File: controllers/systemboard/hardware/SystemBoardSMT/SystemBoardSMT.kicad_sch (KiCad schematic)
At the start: 35 parts, among them J1 5V, J2 5V, J3 JTAG, SW1 RESET, U1 ATF1508AS-xxAx100, U2 74HC14, Y1 Crystal

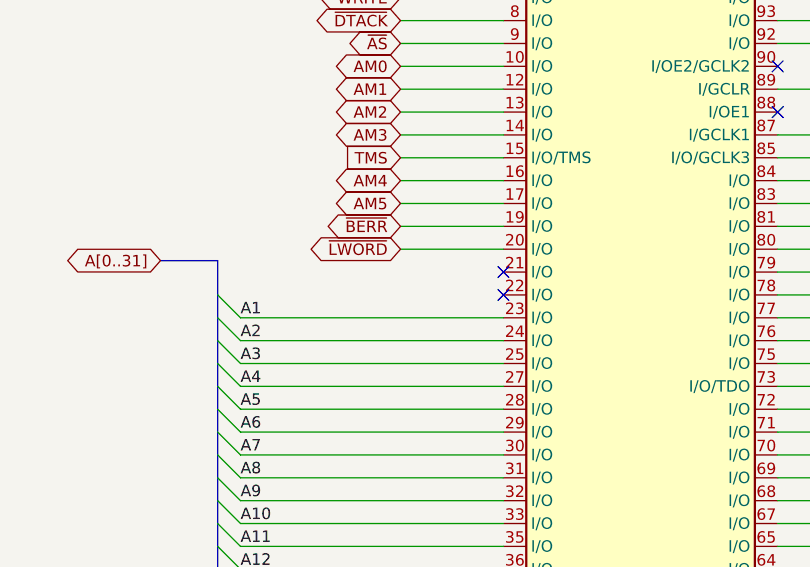
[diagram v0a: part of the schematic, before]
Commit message: Reorganized a bit
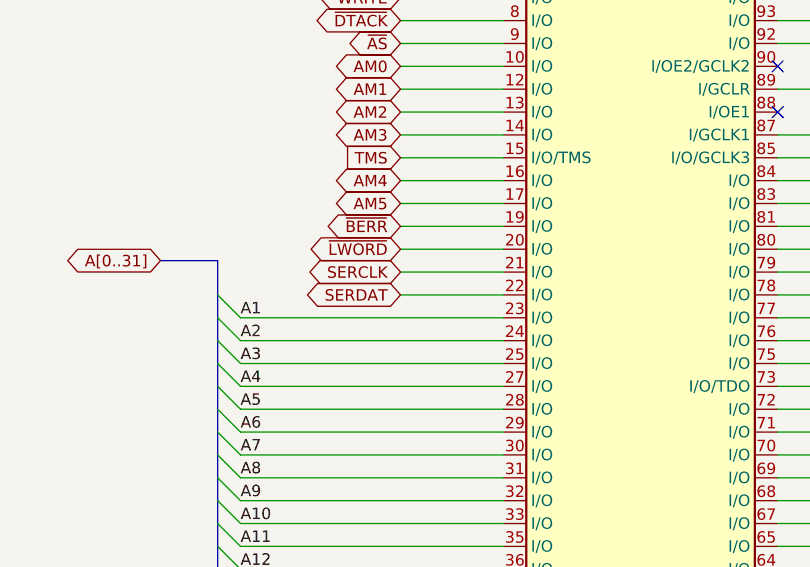
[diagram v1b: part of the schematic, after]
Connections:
- net SERCLK: now reaches U1.21 (I/O)
- net SERDAT: now reaches U1.22 (I/O)
- no-connect marks 16 -> 14
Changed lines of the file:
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@@
 	)
 	(no_connect
-		(at 161.29 88.9)
-	)
-	(no_connect
 		(at 255.27 142.24)
 	)
@@
 		(at 255.27 154.94)
 	)
-	(no_connect
-		(at 161.29 86.36)
-	)
 	(bus_entry
 		(at 132.08 96.52)
@@
 		)
 	)
+	(wire
+		(pts
+			(xy 149.86 88.9) (xy 161.29 88.9)
+		)
+		(stroke
+			(width 0)
+			(type default)
+		)
+	)
 	(bus
 		(pts
@@
 	(wire
 		(pts
+			(xy 149.86 86.36) (xy 161.29 86.36)
+		)
+		(stroke
+			(width 0)
+			(type default)
+		)
+	)
+	(wire
+		(pts
 			(xy 203.2 109.22) (xy 191.77 109.22)
 		)
@@
 		)
 	)
+	(global_label "SERDAT"
+		(shape bidirectional)
+		(at 149.86 88.9 180)
+		(fields_autoplaced yes)
+		(effects
+			(font
+				(size 1.27 1.27)
+			)
+			(justify right)
+		)
+		(property "Intersheetrefs" "${INTERSHEET_REFS}"
+			(at 138.8088 88.9 0)
+			(effects
+				(font
+					(size 1.27 1.27)
+				)
+				(justify right)
+				(hide yes)
+			)
+		)
+	)
 	(global_label "AM3"
 		(shape bidirectional)
@@
 				(hide yes)
 			)
+		)
+	)
+	(global_label "SERCLK"
+		(shape bidirectional)
+		(at 149.86 86.36 180)
+		(fields_autoplaced yes)
+		(effects
+			(font
+				(size 1.27 1.27)
+			)
+			(justify right)
+		)
+		(property "Intersheetrefs" "${INTERSHEET_REFS}"
+			(at 138.5669 86.36 0)
+			(effects
+				(font
+					(size 1.27 1.27)
+				)
+				(justify right)
+				(hide yes)
+			)
